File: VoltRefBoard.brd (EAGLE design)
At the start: 50 x 50 mm, 29 parts, among them J1 BANANA_CONN, J2 BANANA_CONN, J3 BANANA_CONN, J4 BANANA_CONN, J5 BANANA_CONN, U1 MAX6225ACSA+, U2 MAX6250ACSA+

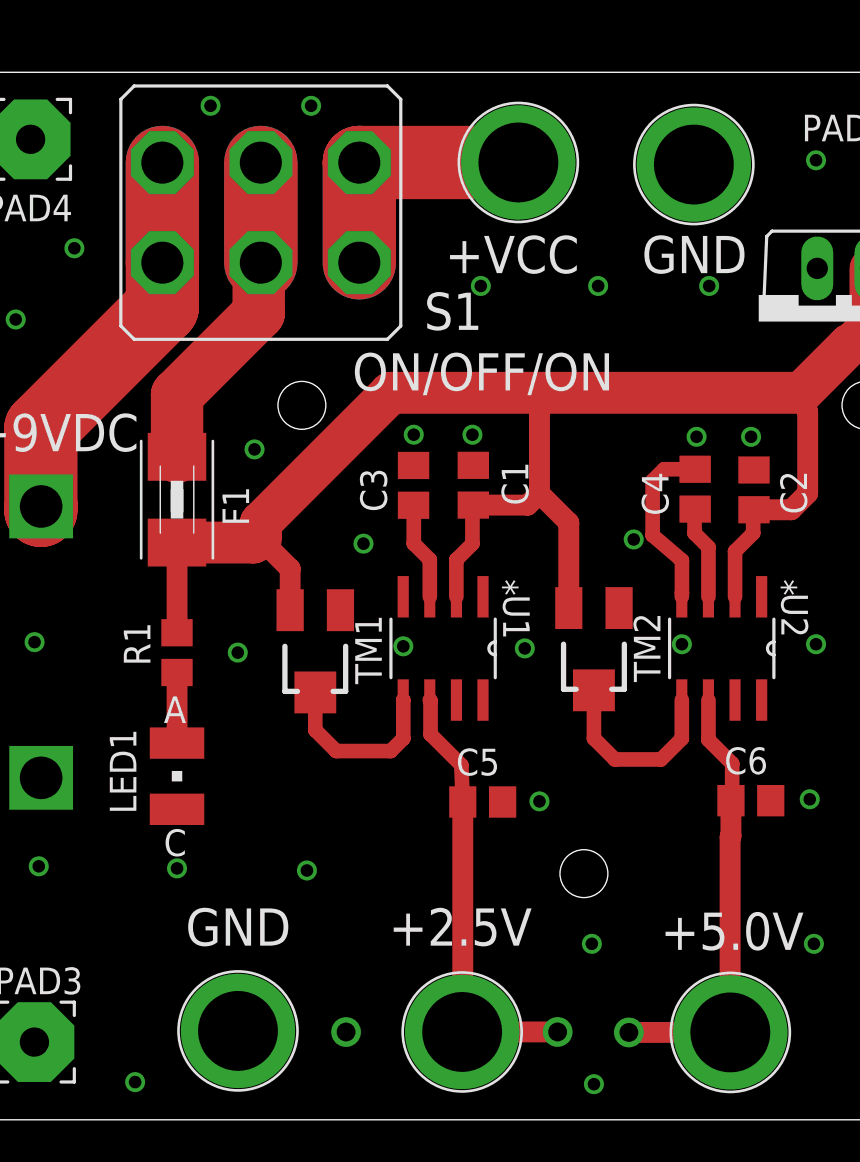
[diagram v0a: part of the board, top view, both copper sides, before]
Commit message: Latest commits
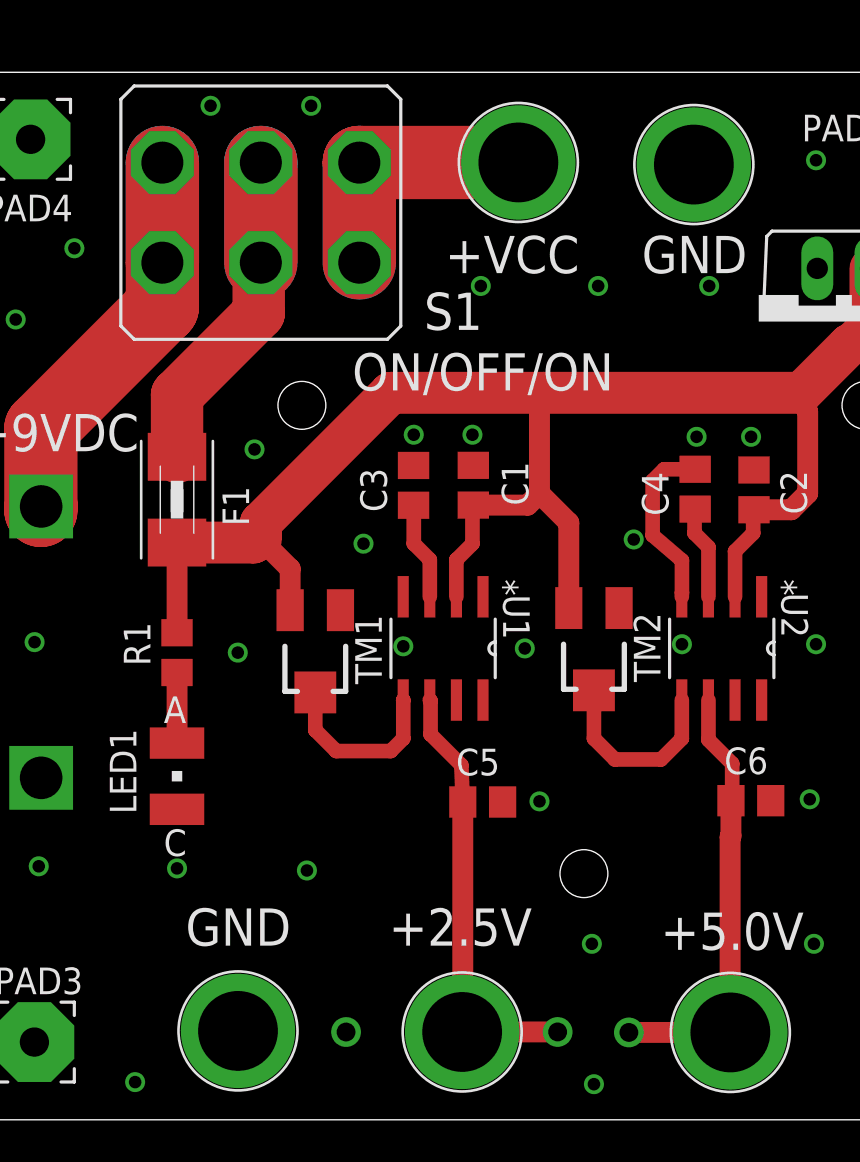
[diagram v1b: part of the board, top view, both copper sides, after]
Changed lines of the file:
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@@
 <setting verticaltext="up"/>
 </settings>
-<grid distance="0.1" unitdist="mm" unit="mm" style="lines" multiple="1" display="no" altdistance="0.05" altunitdist="mm" altunit="mm"/>
+<grid distance="0.00393700787" unitdist="inch" unit="inch" style="lines" multiple="1" display="no" altdistance="0.00196850394" altunitdist="inch" altunit="inch"/>
 <layers>
 <layer number="1" name="Top" color="4" fill="1" visible="yes" active="yes"/>
@@
 </element>
 <element name="TP1" library="TP_1MM_TH" package="TP_1MM_TH" value="TP_1MM_TH&quot;" x="28.5675" y="4.1925">
-<attribute name="OC_FARNELL" value="unknown" x="28.5675" y="4.1925" size="1.778" layer="27" display="off"/>
-<attribute name="MF" value="" x="28.5675" y="4.1925" size="1.778" layer="27" display="off"/>
-<attribute name="MPN" value="" x="28.5675" y="4.1925" size="1.778" layer="27" display="off"/>
+<attribute name="OC_FARNELL" value="1702006" x="28.5675" y="4.1925" size="1.778" layer="27" display="off"/>
+<attribute name="MF" value="MULTICOMP" x="28.5675" y="4.1925" size="1.778" layer="27" display="off"/>
+<attribute name="MPN" value="TEST-3" x="28.5675" y="4.1925" size="1.778" layer="27" display="off"/>
 </element>
 <element name="TP3" library="TP_1MM_TH" package="TP_1MM_TH" value="TP_1MM_TH&quot;" x="18.4675" y="4.19">
-<attribute name="OC_FARNELL" value="unknown" x="18.4675" y="4.19" size="1.778" layer="27" display="off"/>
-<attribute name="MF" value="" x="18.4675" y="4.19" size="1.778" layer="27" display="off"/>
-<attribute name="MPN" value="" x="18.4675" y="4.19" size="1.778" layer="27" display="off"/>
+<attribute name="OC_FARNELL" value="1702006" x="18.4675" y="4.19" size="1.778" layer="27" display="off"/>
+<attribute name="MF" value="MULTICOMP" x="18.4675" y="4.19" size="1.778" layer="27" display="off"/>
+<attribute name="MPN" value="TEST-3" x="18.4675" y="4.19" size="1.778" layer="27" display="off"/>
 </element>
 <element name="C2" library="rcl" package="C0805" value="2.2uF" x="37.94" y="30.0675" smashed="yes" rot="R90">
@@
 </element>
 <element name="TP2" library="TP_1MM_TH" package="TP_1MM_TH" value="TP_1MM_TH&quot;" x="31.9675" y="4.17">
-<attribute name="OC_FARNELL" value="unknown" x="31.9675" y="4.17" size="1.778" layer="27" display="off"/>
-<attribute name="MF" value="" x="31.9675" y="4.17" size="1.778" layer="27" display="off"/>
-<attribute name="MPN" value="" x="31.9675" y="4.17" size="1.778" layer="27" display="off"/>
+<attribute name="OC_FARNELL" value="1702006" x="31.9675" y="4.17" size="1.778" layer="27" display="off"/>
+<attribute name="MF" value="MULTICOMP" x="31.9675" y="4.17" size="1.778" layer="27" display="off"/>
+<attribute name="MPN" value="TEST-3" x="31.9675" y="4.17" size="1.778" layer="27" display="off"/>
 </element>
 <element name="PAD1" library="wirepad" package="3,81/1,4" value="MOUNT_HOLE" x="46.7225" y="46.6175" smashed="yes">
@@
 </element>
 <element name="LED1" library="P-LCC-2_Shorter" package="P-LCC-2" value="GREEN_LED" x="10.4" y="16.4" smashed="yes">
-<attribute name="MPN" value="" x="1.7" y="30.4" size="1.778" layer="27" display="off"/>
-<attribute name="MF" value="" x="1.7" y="30.4" size="1.778" layer="27" display="off"/>
-<attribute name="OC_FARNELL" value="unknown" x="1.7" y="30.4" size="1.778" layer="27" display="off"/>
+<attribute name="MPN" value="LGT67K-H2K1-24-Z" x="1.7" y="30.4" size="1.778" layer="27" display="off"/>
+<attribute name="MF" value="OSRAM" x="1.7" y="30.4" size="1.778" layer="27" display="off"/>
+<attribute name="OC_FARNELL" value="1226376" x="1.7" y="30.4" size="1.778" layer="27" display="off"/>
 <attribute name="NAME" x="8.46" y="14.595" size="1.27" layer="25" rot="R90"/>
 <attribute name="VALUE" x="14.21" y="14.495" size="1.27" layer="27" rot="R90"/>
@@
 </element>
 <element name="TM1" library="P-LCC-2_Shorter" package="TC33X" value="10k" x="17" y="22.2" rot="R180">
-<attribute name="OC_FARNELL" value="unknown" x="17" y="22.2" size="1.778" layer="27" rot="R180" display="off"/>
-<attribute name="MF" value="" x="17" y="22.2" size="1.778" layer="27" rot="R180" display="off"/>
-<attribute name="MPN" value="" x="17" y="22.2" size="1.778" layer="27" rot="R180" display="off"/>
+<attribute name="OC_FARNELL" value="1141485" x="17" y="22.2" size="1.778" layer="27" rot="R180" display="off"/>
+<attribute name="MF" value="VISHAY SFERNICE" x="17" y="22.2" size="1.778" layer="27" rot="R180" display="off"/>
+<attribute name="MPN" value="TS53YJ103MR10" x="17" y="22.2" size="1.778" layer="27" rot="R180" display="off"/>
 </element>
 <element name="TM2" library="P-LCC-2_Shorter" package="TC33X" value="10k" x="30.3" y="22.3" rot="R180">
-<attribute name="OC_FARNELL" value="unknown" x="30.3" y="22.3" size="1.778" layer="27" rot="R180" display="off"/>
-<attribute name="MF" value="" x="30.3" y="22.3" size="1.778" layer="27" rot="R180" display="off"/>
-<attribute name="MPN" value="" x="30.3" y="22.3" size="1.778" layer="27" rot="R180" display="off"/>
+<attribute name="OC_FARNELL" value="1141485" x="30.3" y="22.3" size="1.778" layer="27" rot="R180" display="off"/>
+<attribute name="MF" value="VISHAY SFERNICE" x="30.3" y="22.3" size="1.778" layer="27" rot="R180" display="off"/>
+<attribute name="MPN" value="TS53YJ103MR10" x="30.3" y="22.3" size="1.778" layer="27" rot="R180" display="off"/>
 </element>
 <element name="F1" library="adafruit" package="1812" value="1.1A" x="10.4" y="29.6" smashed="yes" rot="R90">
@@
 <wire x1="36.8" y1="13.5" x2="36.8" y2="4.18" width="1" layer="1"/>
 <wire x1="31.9675" y1="4.17" x2="36.81" y2="4.17" width="1" layer="1"/>
-<wire x1="36.81" y1="4.17" x2="36.8" y2="4.18" width="0" layer="19" extent="1-1"/>
+<wire x1="36.81" y1="4.17" x2="36.8" y2="4.17" width="0.4064" layer="1"/>
+<wire x1="36.8" y1="4.17" x2="36.8" y2="4.18" width="0.4064" layer="1"/>
 </signal>
 <signal name="V_IN_A">
@@
 <contactref element="S1" pad="6"/>
 <wire x1="19.1" y1="45.6876" x2="19.1" y2="40.9124" width="3.5" layer="1"/>
-<wire x1="19.1" y1="45.7" x2="19.1" y2="40.9" width="3.5" layer="16"/>
+<wire x1="19.1" y1="45.7" x2="19.1" y2="45.6876" width="3.5" layer="16"/>
 <contactref element="J1" pad="P$1"/>
+<wire x1="19.1" y1="45.6876" x2="19.1" y2="40.9" width="3.5" layer="16"/>
 <wire x1="26.6925" y1="45.695" x2="19.1074" y2="45.695" width="3.5" layer="1"/>
 <wire x1="19.1074" y1="45.695" x2="19.1" y2="45.6876" width="3.5" layer="1"/>
-<wire x1="19.1" y1="45.7" x2="19.1074" y2="45.695" width="0" layer="19" extent="1-16"/>
 </signal>
 <signal name="V_IN_B">
@@
 <wire x1="3.9" y1="29.09" x2="3.914" y2="29.276" width="3.5" layer="1"/>
 <wire x1="9.7" y1="40.9124" x2="9.7" y2="45.6876" width="3.5" layer="1"/>
-<wire x1="9.7" y1="45.7" x2="9.7" y2="40.9" width="3.5" layer="16"/>
+<wire x1="9.7" y1="45.7" x2="9.7" y2="45.6876" width="3.5" layer="16"/>
+<wire x1="9.7" y1="45.6876" x2="9.7" y2="40.9" width="3.5" layer="16"/>
 <wire x1="9.7" y1="40.9124" x2="9.7" y2="38.8" width="3.5" layer="1"/>
 <wire x1="9.7" y1="38.8" x2="3.9" y2="33" width="3.5" layer="1"/>
-<wire x1="9.7" y1="45.6876" x2="9.7" y2="45.7" width="0" layer="19" extent="16-16"/>
 </signal>
 <signal name="N$30">
@@
 <contactref element="F1" pad="2"/>
 <wire x1="14.4" y1="45.6876" x2="14.4" y2="40.9124" width="3.5" layer="1"/>
-<wire x1="14.4" y1="45.7" x2="14.4" y2="40.9" width="3.5" layer="16"/>
+<wire x1="14.4" y1="45.7" x2="14.4" y2="45.6876" width="3.5" layer="16"/>
+<wire x1="14.4" y1="45.6876" x2="14.4" y2="40.9" width="3.5" layer="16"/>
 <wire x1="10.4" y1="31.646" x2="10.4" y2="34.6" width="2.5" layer="1"/>
 <wire x1="10.4" y1="34.6" x2="14.3" y2="38.5" width="2.5" layer="1"/>
 <wire x1="14.3" y1="38.5" x2="14.3" y2="40.8124" width="2.5" layer="1"/>
 <wire x1="14.3" y1="40.8124" x2="14.4" y2="40.9124" width="2.5" layer="1"/>
-<wire x1="14.4" y1="45.6876" x2="14.4" y2="45.7" width="0" layer="19" extent="16-16"/>
 </signal>
 <signal name="N$4">
